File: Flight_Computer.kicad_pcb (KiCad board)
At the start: 4 copper layers, 75.8 x 76.2 mm, 145 parts, among them IC1 PIC32MZ2048EFH144-I_PL, IC2 FAN4010IL6X_F113, IC3 FAN4010IL6X_F113, J1 ICSP Programming, J2 SC_19-20, J3 UJ2-MBH-1-SMT-TR, J4 47219-2001, Q1 Q_NPN_BEC, Q2 Q_NPN_BEC, U1 STMPS2141STR, U2 STMPS2141STR, U3 BNO055, U4 SN65HVD1050D, U5 SN74LVC1T45DBVR, U6 SN74LVC1T45DBVR, U8 TXB0104PWR

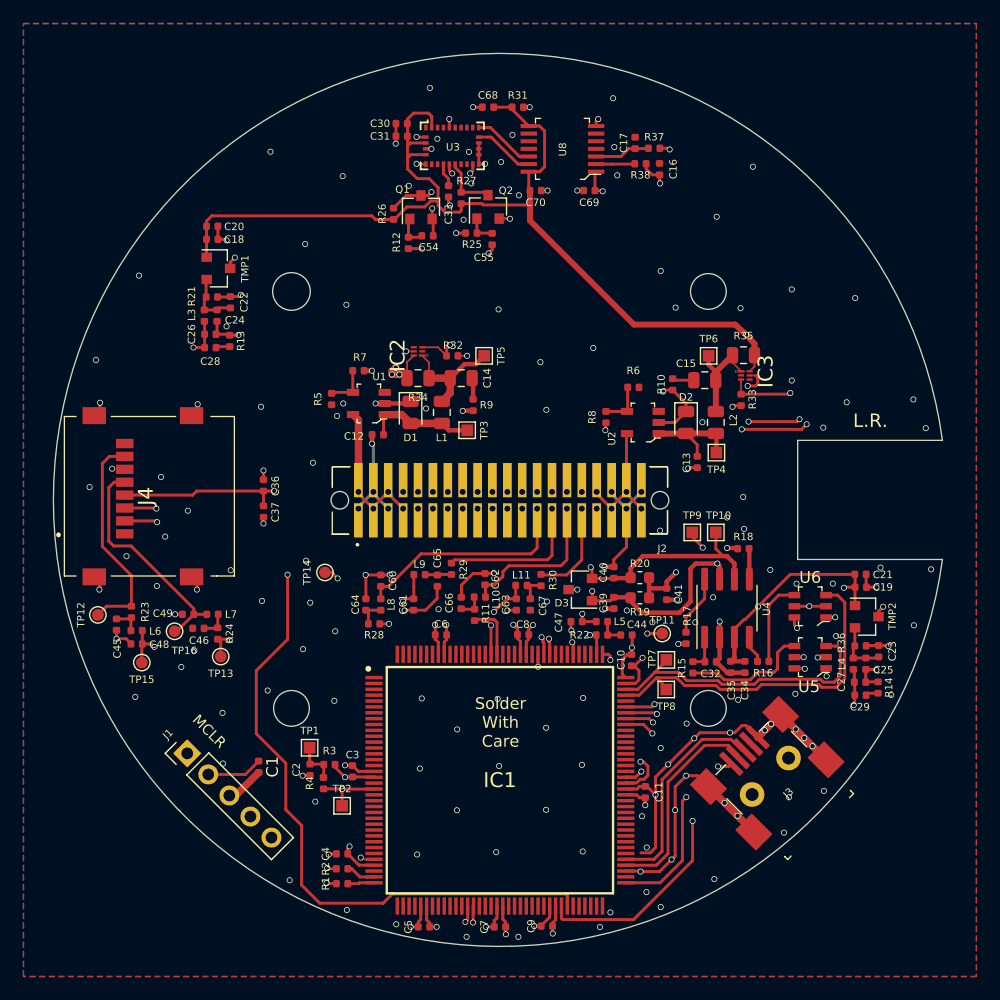
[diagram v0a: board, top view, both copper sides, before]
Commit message: Fixed Vias
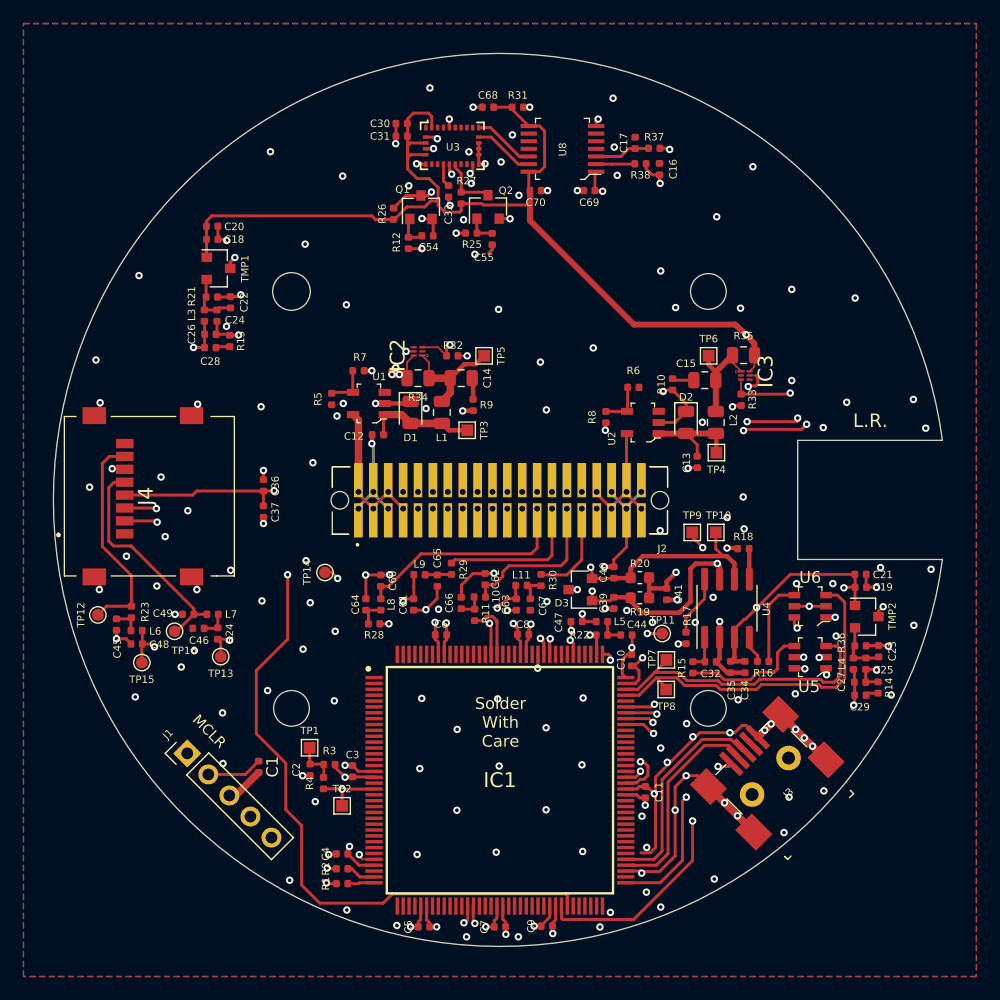
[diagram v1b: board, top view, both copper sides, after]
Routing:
- net GND: track 176.7 -> 175.4 mm, vias 189 -> 187
- net BNO_BL_IND: vias 3 -> 2
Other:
- net class Default: via_dia 0.508 -> 0.635; via_drill 0.381 -> 0.3048
- rule trace_min: 0.127 -> 0
- rule via_min_size: 0.3048 -> 0.635
